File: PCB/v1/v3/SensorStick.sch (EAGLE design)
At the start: 73 parts, among them U1 TPD4F003DQDR, Y1 ECS-TXO-3225MV-400-TR

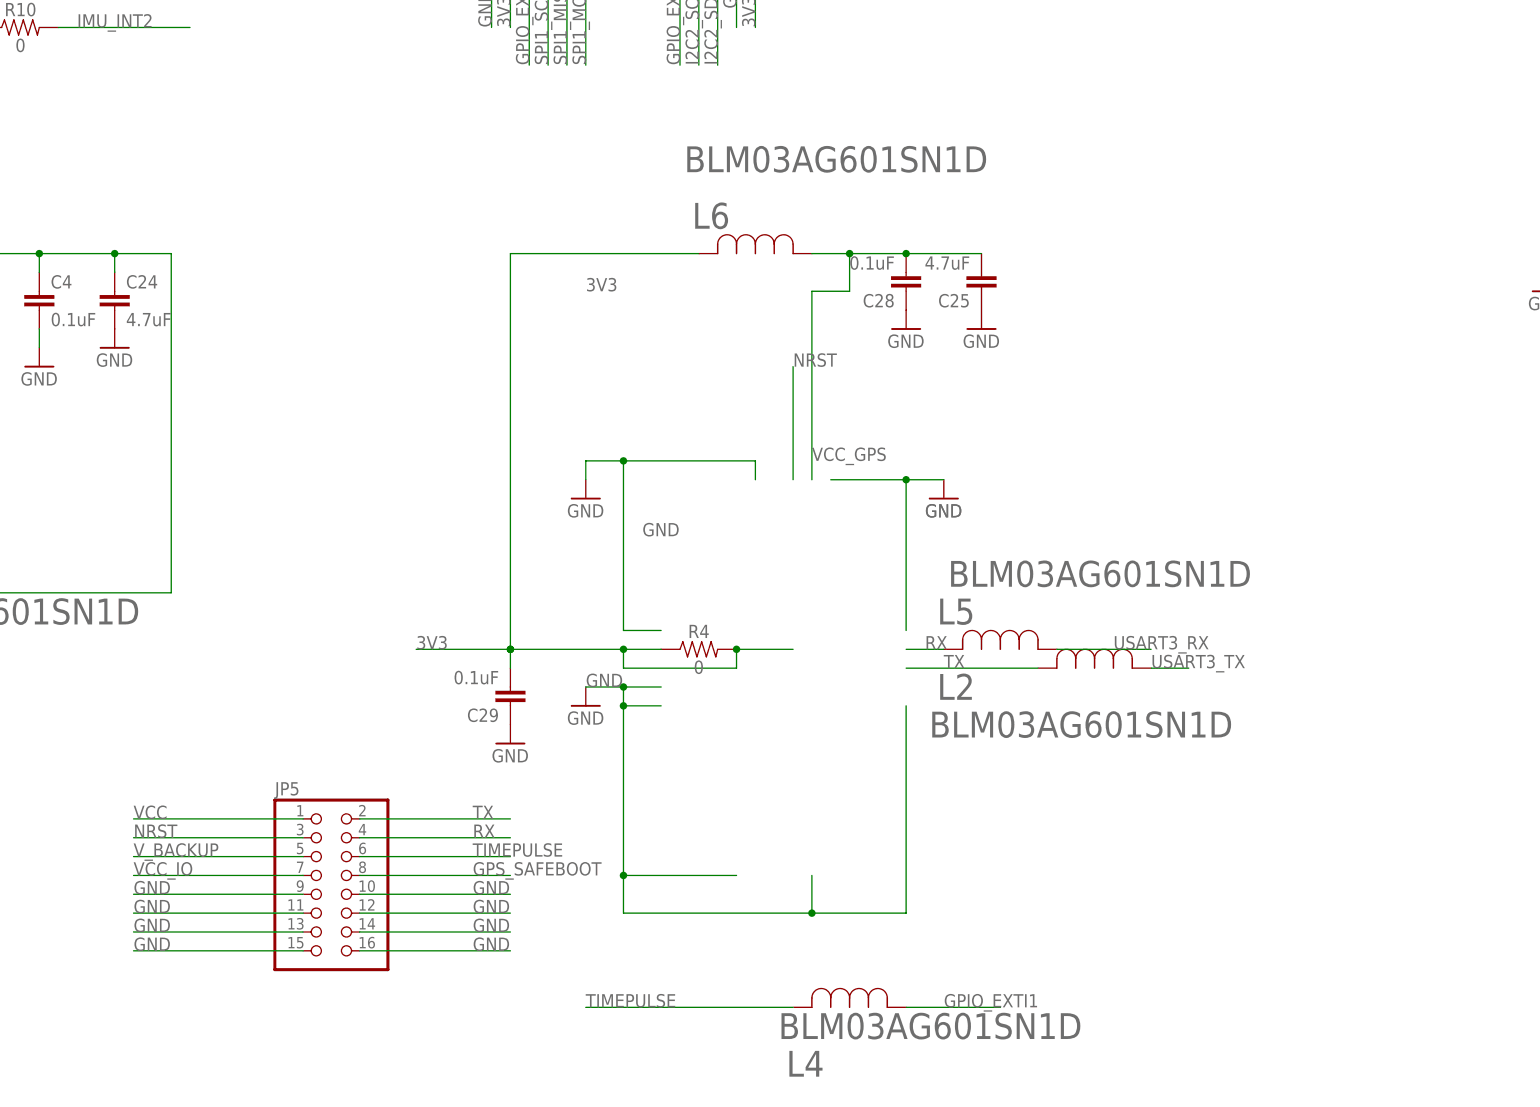
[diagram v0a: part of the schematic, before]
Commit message: Jesus - Cleaning up GPS schematic
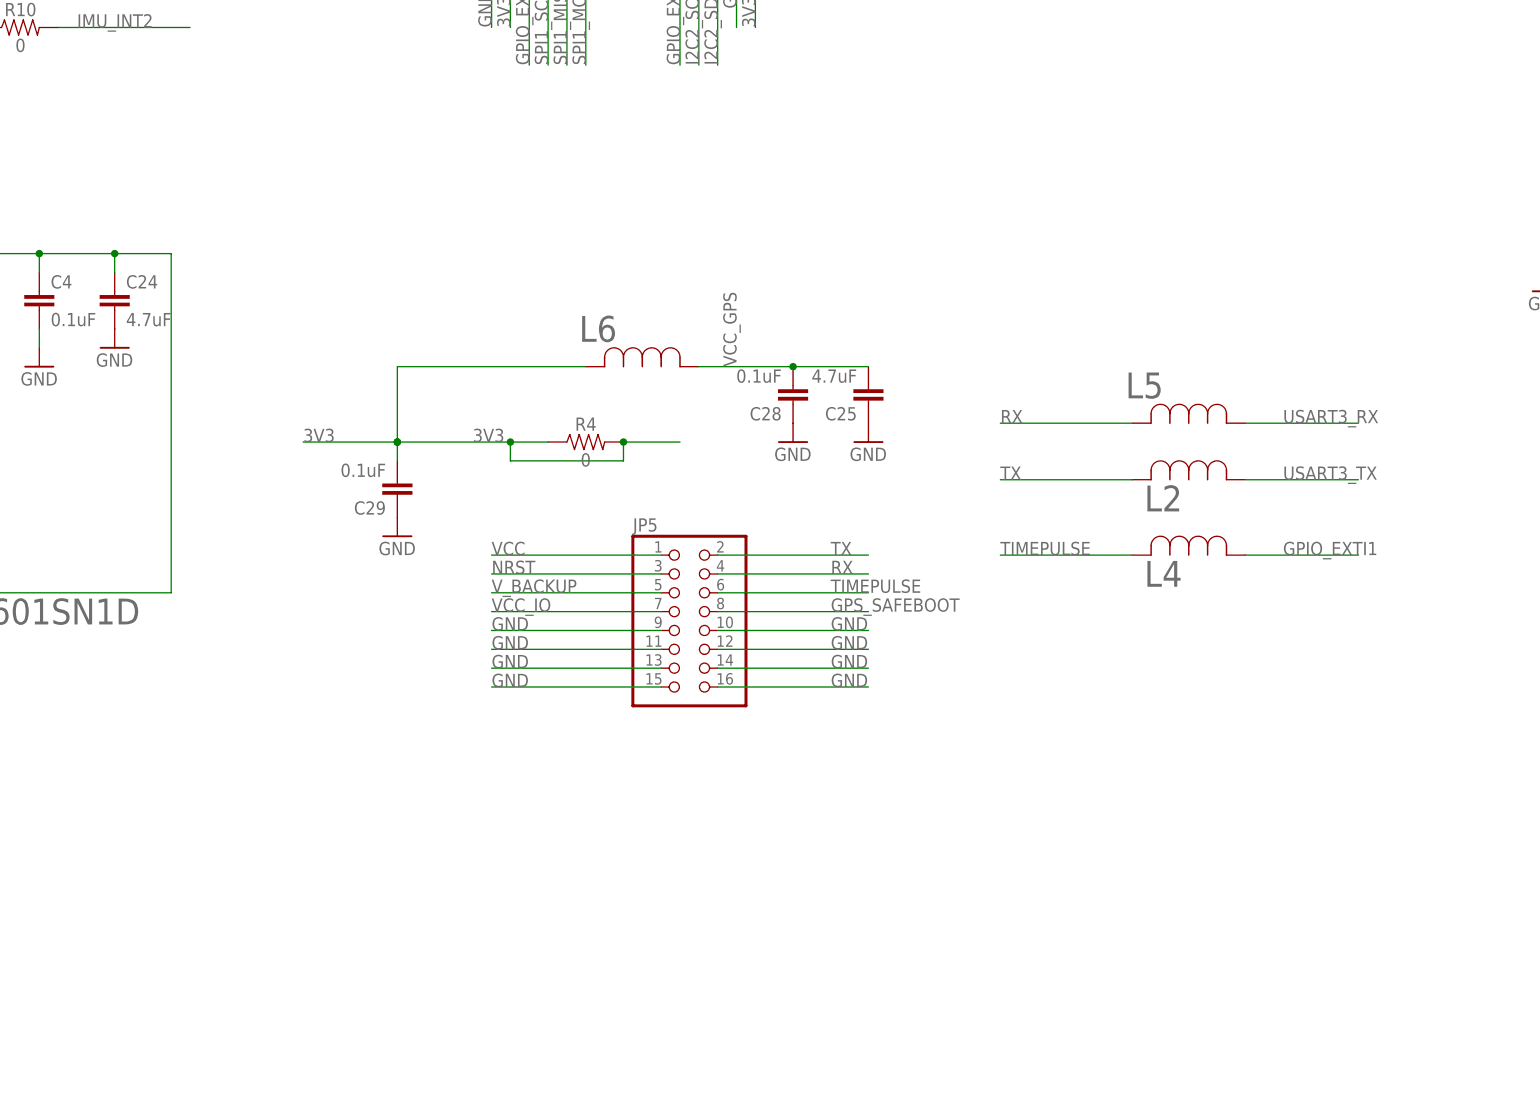
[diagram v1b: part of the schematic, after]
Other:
- moved on the sheet: C25, C28, C29, JP5, L2, L4, L5, L6, R4
